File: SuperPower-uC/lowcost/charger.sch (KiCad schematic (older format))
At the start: 17 parts, among them J2 Thermistor, Q2 2N7002, U3 LC709203FQH, U4 TP4056

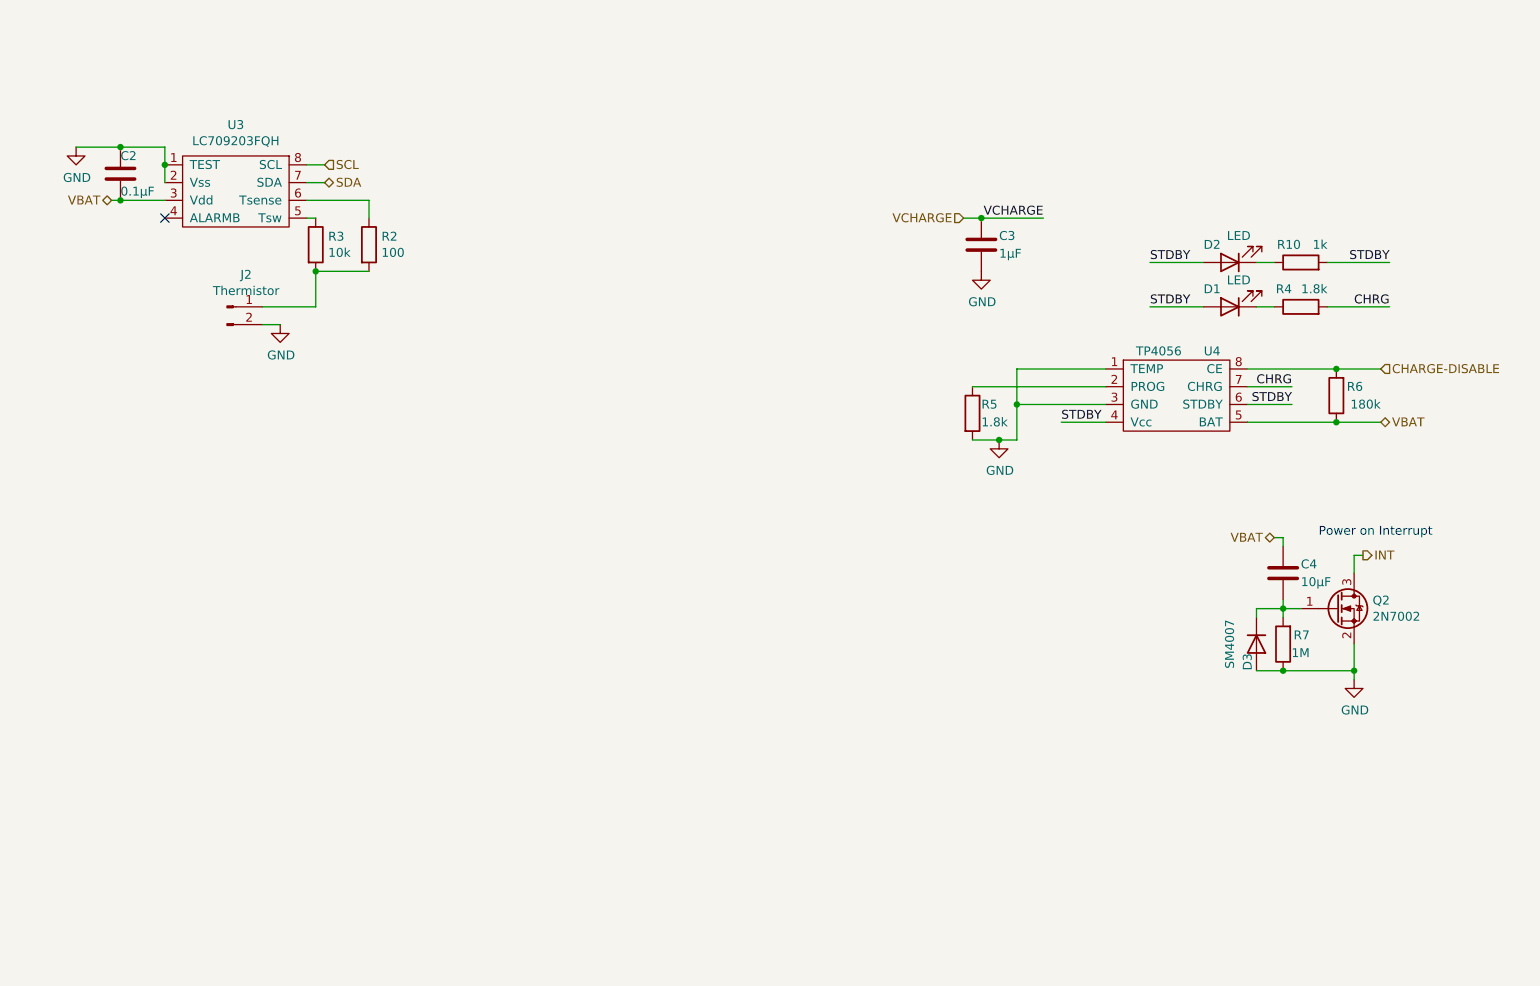
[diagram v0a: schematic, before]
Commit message: schematic layout cleaning
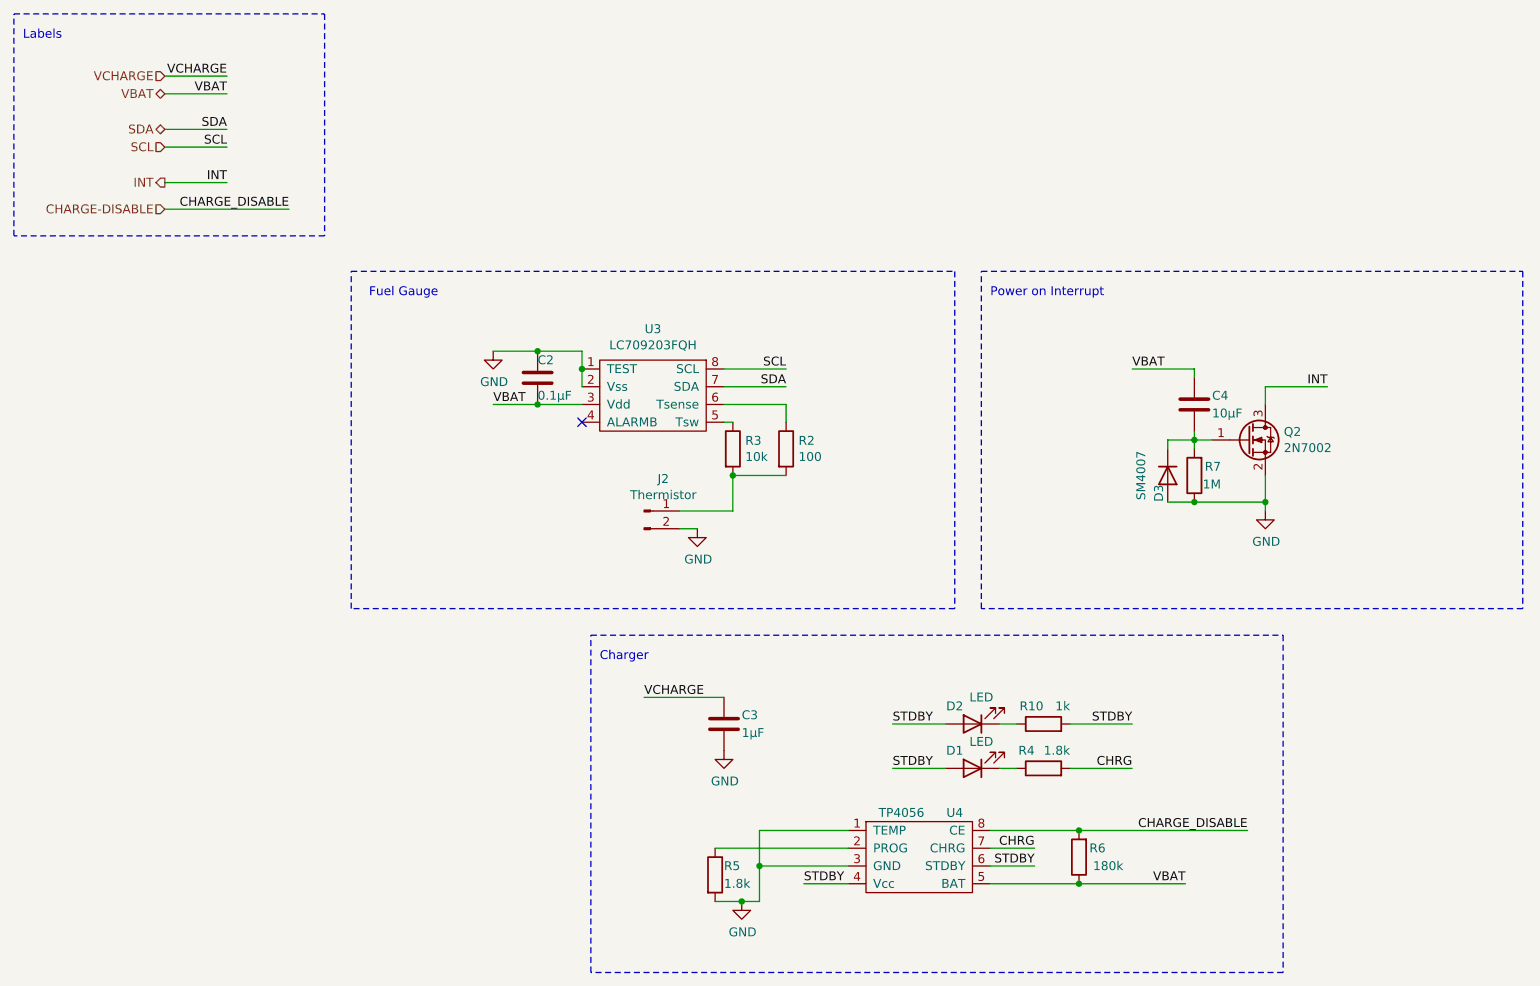
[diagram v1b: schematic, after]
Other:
- note added: "Charger\n"
- note added: "Fuel Gauge"
- note added: "Labels\n"
- moved on the sheet: C2, C3, C4, D1, D2, D3, J2, Q2, R10, R2, R3, R4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
